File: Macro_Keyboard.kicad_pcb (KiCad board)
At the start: 4 copper layers, 95.6 x 84.2 mm, 115 parts, among them J1 USB_C_Receptacle_USB2.0, J2 USB_A, J3 USB_A, J4 USB_A, SW1 SW_Push, SW10 SW_DIP_x01, SW2 SW_DIP_x01, SW3 SW_DIP_x01, SW4 SW_DIP_x01, SW5 SW_DIP_x01, SW6 SW_DIP_x01, SW7 SW_DIP_x01, SW8 SW_DIP_x01, SW9 SW_DIP_x01, U1 STM32L432KCUx, U2 LD39050PU33R, U5 SRV05-4, U6 SRV05-4, Y1 12MHz

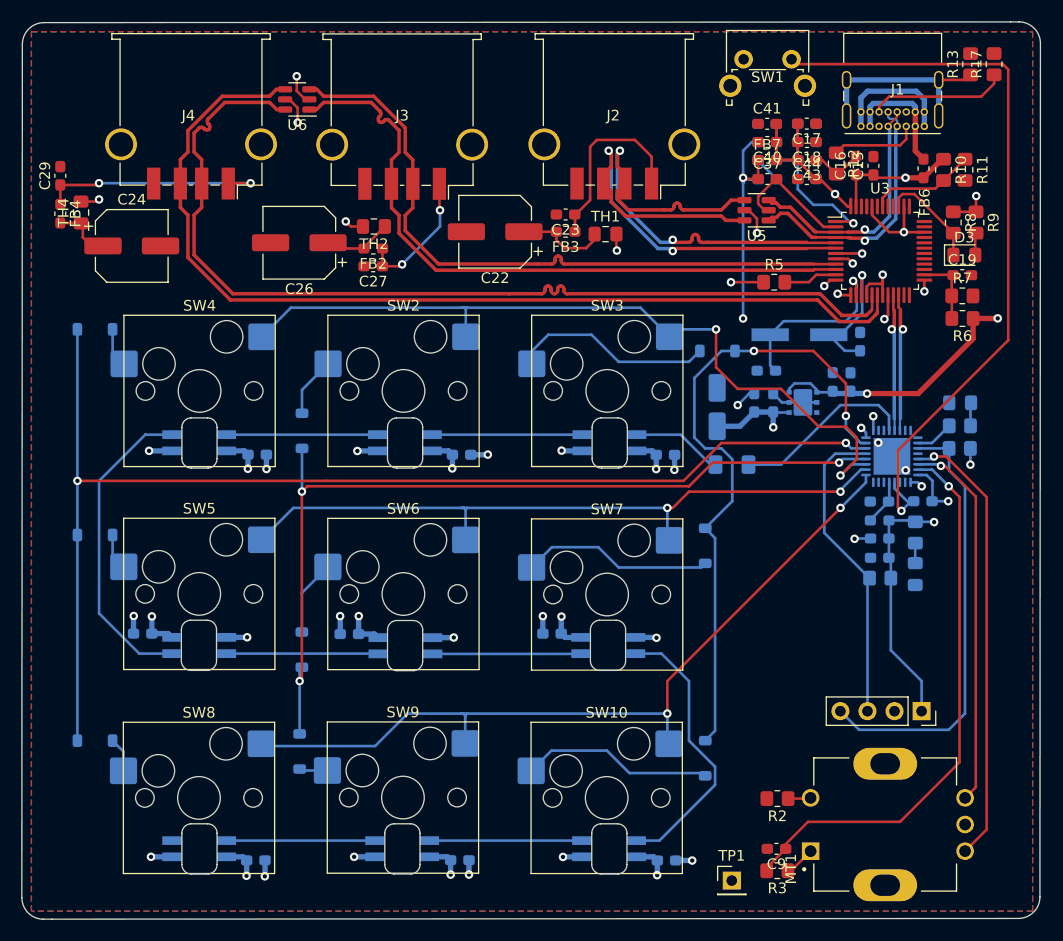
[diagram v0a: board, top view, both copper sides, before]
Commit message: Add files via upload
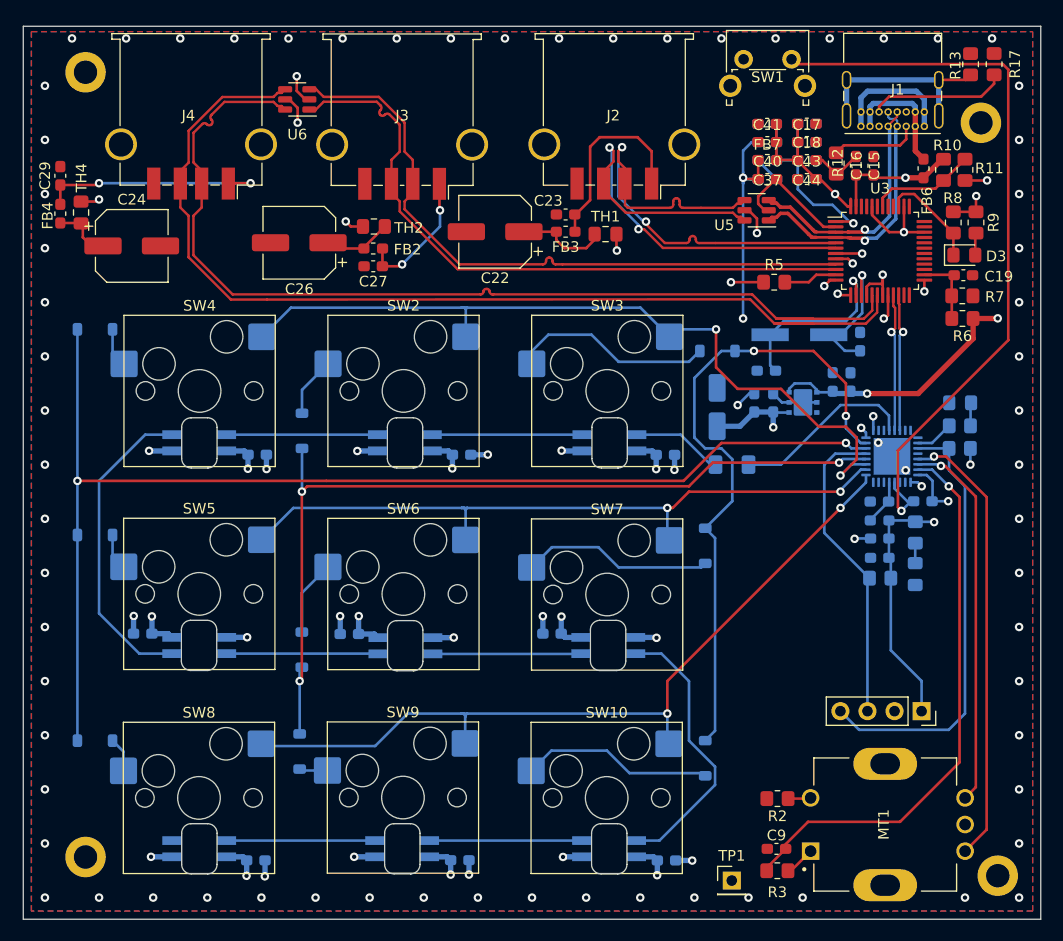
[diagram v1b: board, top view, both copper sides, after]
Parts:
- added ?: , , F.Cu at (67.3, 118.1)
- added ?: , , F.Cu at (152.9, 119.9)
- added ?: , , F.Cu at (67.3, 44.5)
- added ?: , , F.Cu at (151.4, 49.2)
- moved C19 0.10 mm to (149.7, 63.5)
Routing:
- net /USB/D_P3: track 92.4 -> 96.1 mm
- net /USB/D_N3: track 92.3 -> 94.9 mm
- net GND: track 88.0 -> 90.3 mm, vias 20 -> 86
- net /USB/D_P1: track 46.7 -> 47.9 mm
- net /USB/D_N1: track 46.6 -> 47.5 mm
- net Net-(J2-VBUS): track 17.8 -> 18.4 mm
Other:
- board size 95.6 x 84.2 mm -> 95.5 x 83.8 mm
- board text added: "Stundner 2023 Macro Keyboard Rev. 0.7"
- board text removed: "Orientation from LEDS Note Add !!!"
